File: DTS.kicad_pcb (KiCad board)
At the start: 2 copper layers, 157 x 122.5 mm, 93 parts, among them J1 Conn_01x02_Pin, J2 Conn_01x06_Pin, J3 Conn_01x02_Pin, J4 Conn_01x06_Pin, SW1 SW_DIP_x01, SW2 SW_DIP_x01, SW3 SW_DIP_x01, SW4 SW_DIP_x01, SW5 SW_DIP_x01, SW6 SW_DIP_x01, SW7 SW_DIP_x01, SW8 SW_DIP_x01, SW9 SW_DIP_x01, U1 4081, U10 4071, U11 4081, U12 4081, U13 4071, U14 4069, U15 4081, U16 4081, U17 4071, U18 4069, U19 4081, U2 4081, U20 4081, U21 4071, U22 4069, U23 4081, U24 4081, U25 4081, U26 4071, U27 4069, U28 4081, U29 4081, U3 4071, U30 4081, U31 4071, U32 4069, U34 4081, U35 4081, U36 4071, U37 4069, U38 4081, U39 4081, U4 4069, U40 4071, U41 4081, U42 4081, U43 4071, U44 4081, U45 4081, U46 4071, U47 4081, U48 4081, U49 LM7805_TO220, U5 4069, U6 4081, U7 4081, U8 4071, U9 4069

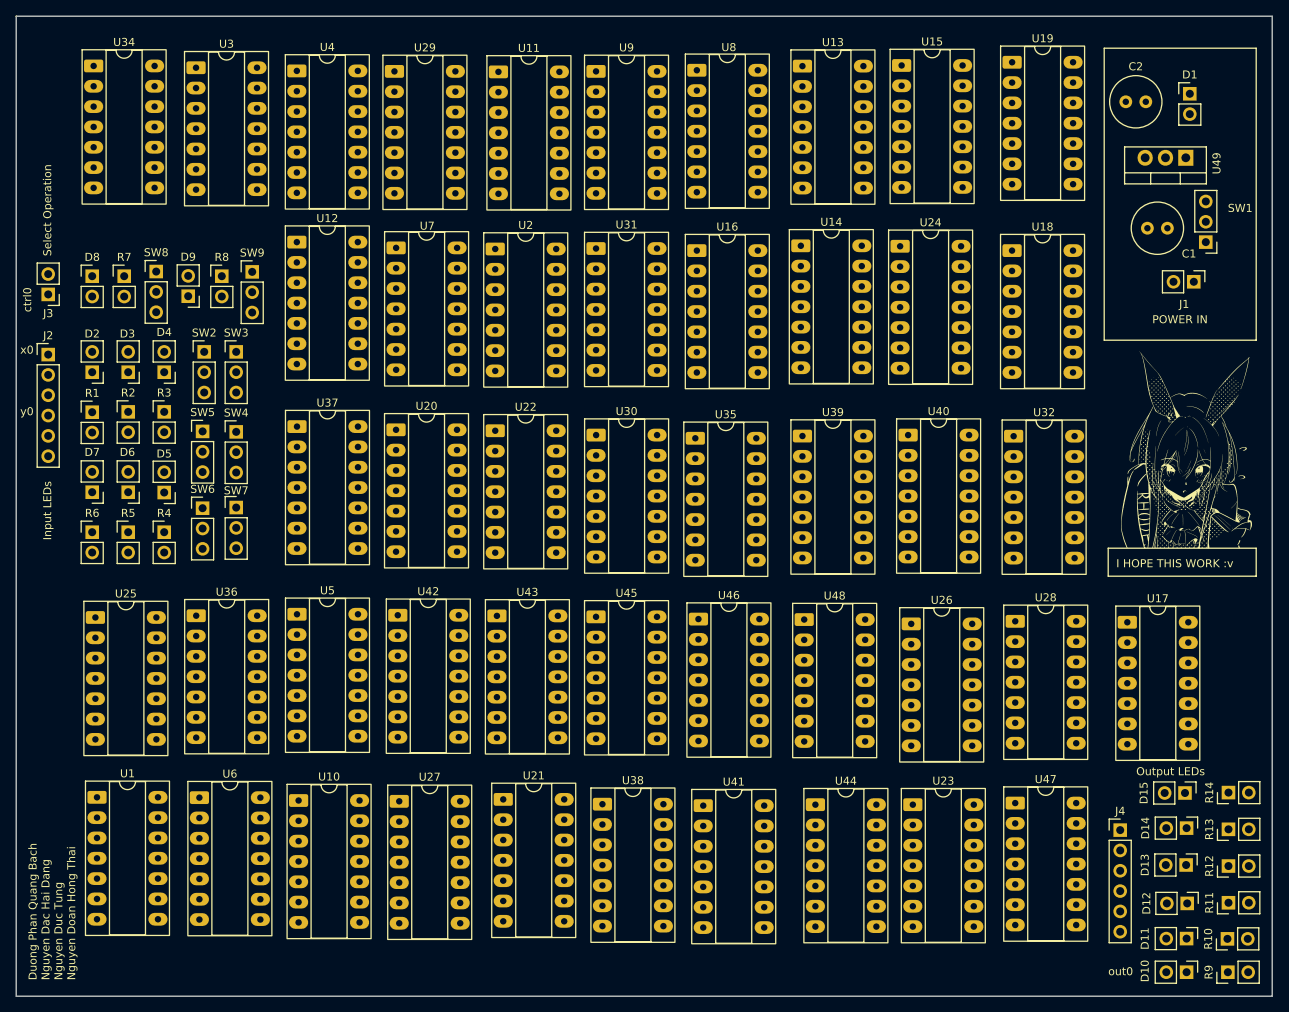
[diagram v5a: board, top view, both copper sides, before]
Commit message: Add files via upload
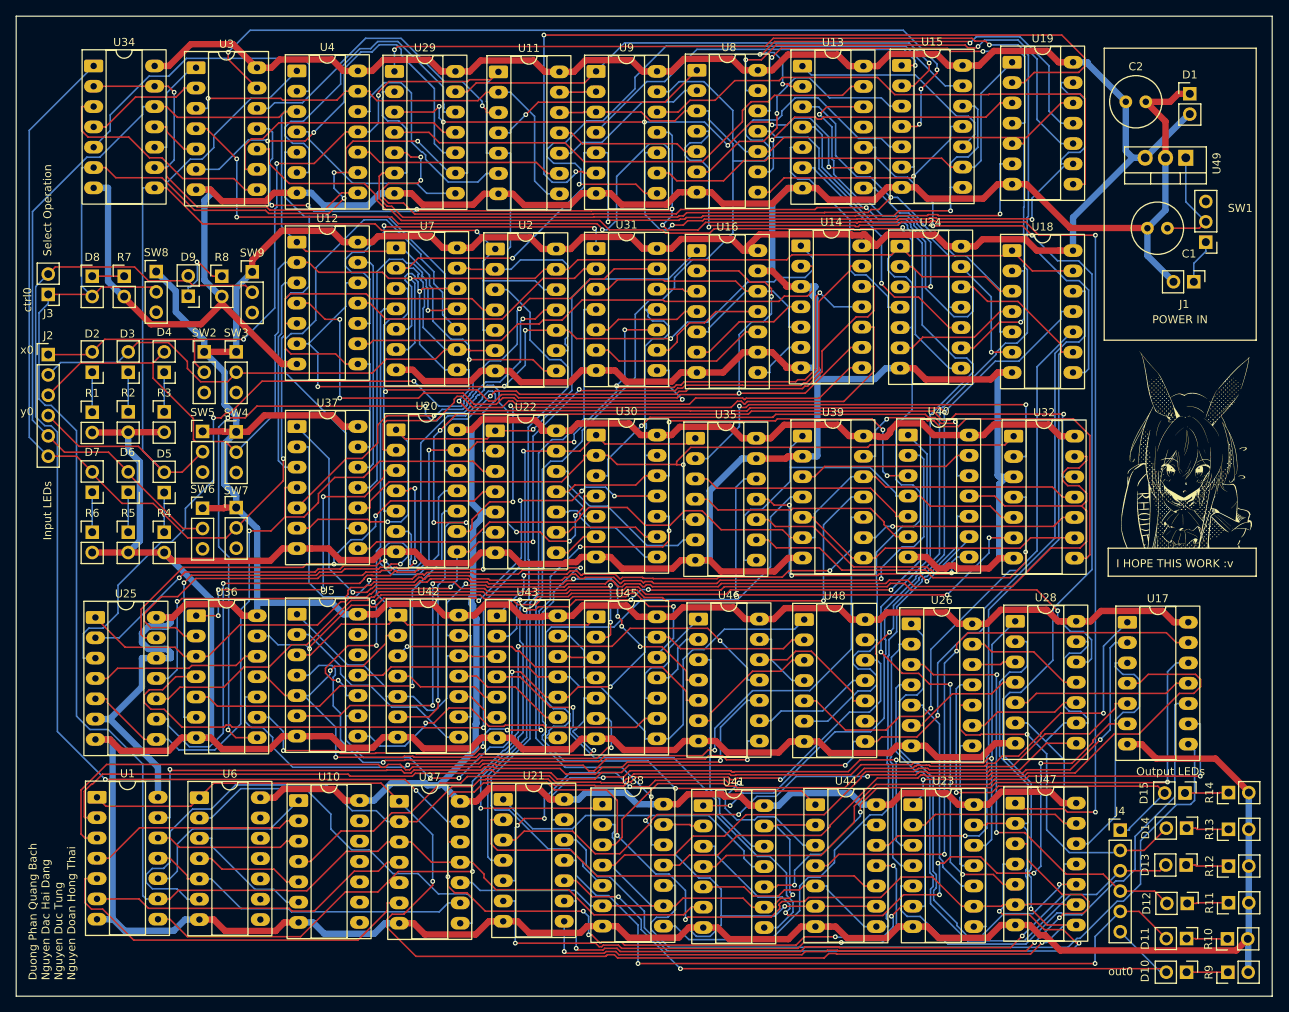
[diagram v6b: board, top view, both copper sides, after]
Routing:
- net GND: track 0.00 -> 915.2 mm
- net VCC: track 0.00 -> 803.1 mm
- net ctrl_out0: track 0.00 -> 411.5 mm, vias 0 -> 5
- net y2: track 0.00 -> 322.5 mm, vias 0 -> 5
- net ctrl_out1: track 0.00 -> 290.2 mm, vias 0 -> 7
- net s2: track 0.00 -> 281.3 mm, vias 0 -> 5
- net x2: track 0.00 -> 256.2 mm, vias 0 -> 1
- net xor2: track 0.00 -> 252.2 mm, vias 0 -> 4
- net x1: track 0.00 -> 183.2 mm, vias 0 -> 3
- net /Signed_Extended/A2': track 0.00 -> 181.7 mm, vias 0 -> 2
- net xor0: track 0.00 -> 172.3 mm, vias 0 -> 2
- net xor1: track 0.00 -> 172.2 mm, vias 0 -> 1
- net y1: track 0.00 -> 155.4 mm, vias 0 -> 1
- net y0: track 0.00 -> 154.1 mm, vias 0 -> 1
- net s0: track 0.00 -> 149.7 mm, vias 0 -> 3
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
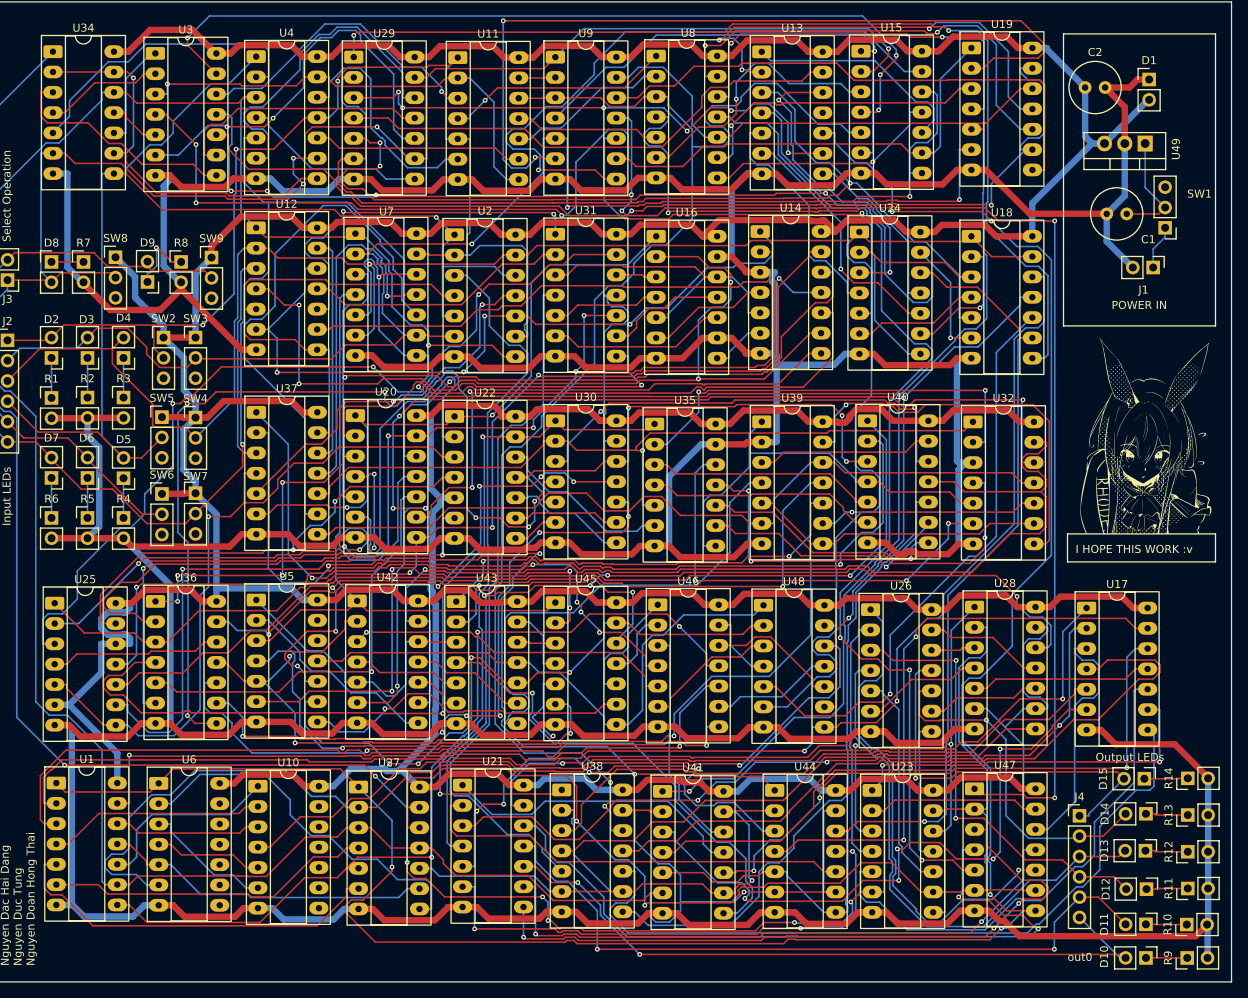
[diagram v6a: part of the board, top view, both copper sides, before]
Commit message: Add files via upload
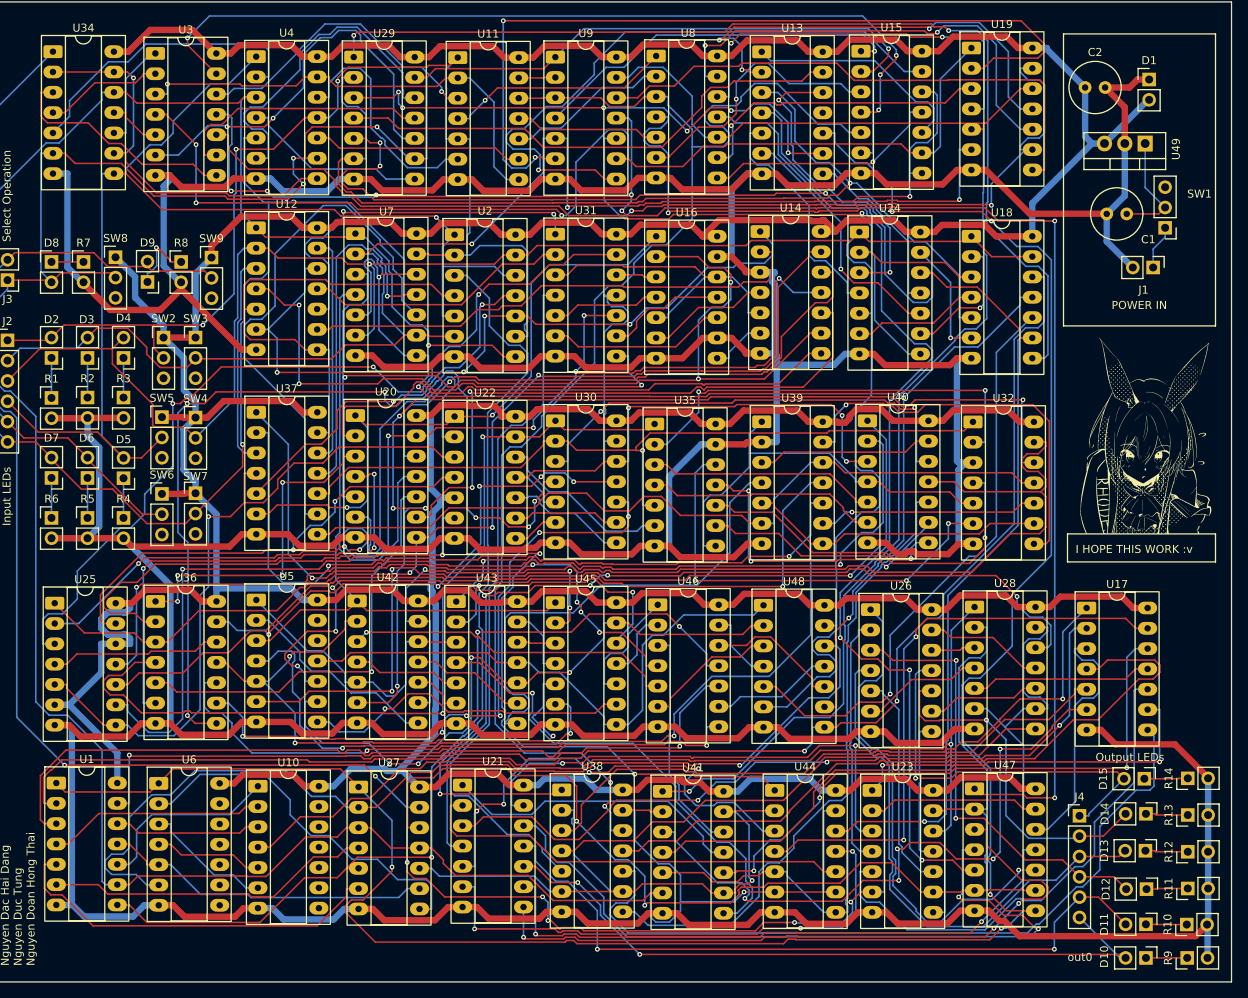
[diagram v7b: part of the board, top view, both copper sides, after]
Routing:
- net ctrl_out0: track 411.5 -> 409.5 mm
- net /Multiplier/cout3: track 74.6 -> 72.7 mm
- net y1: track 155.4 -> 153.8 mm
- net /output 0: track 88.6 -> 87.3 mm
- net x2: track 256.2 -> 255.3 mm
- net GND: track 915.2 -> 914.3 mm
- net /FullAdder/c_out: track 149.2 -> 148.3 mm
- net /mult0: track 90.7 -> 90.0 mm
- net /Multiplexer_6b2/(ctrl)': track 149.4 -> 148.7 mm
- net ctrl_out1: track 290.2 -> 289.6 mm
- net /Multiplexer_3b/temp1: track 13.3 -> 12.7 mm
